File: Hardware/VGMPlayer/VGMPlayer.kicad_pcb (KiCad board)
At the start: 2 copper layers, 94.5 x 103.1 mm, 141 parts, among them J1 Barrel_Jack_Switch, J2 Conn_01x20_Male, J3 Conn_01x20_Male, J4 Conn_01x20_Male, J5 Conn_01x20_Male, U1 STC8951, U10 LTC6903, U11 HC-06, U2 7805-VGM, U3 LM386, U4 LM386, U5 OLED_128_64_I2C, U6 AUDIOJACK-VGM, U7 YM2612, U8 SN76489, U9 LTC6903, Y1 11.0592MHz

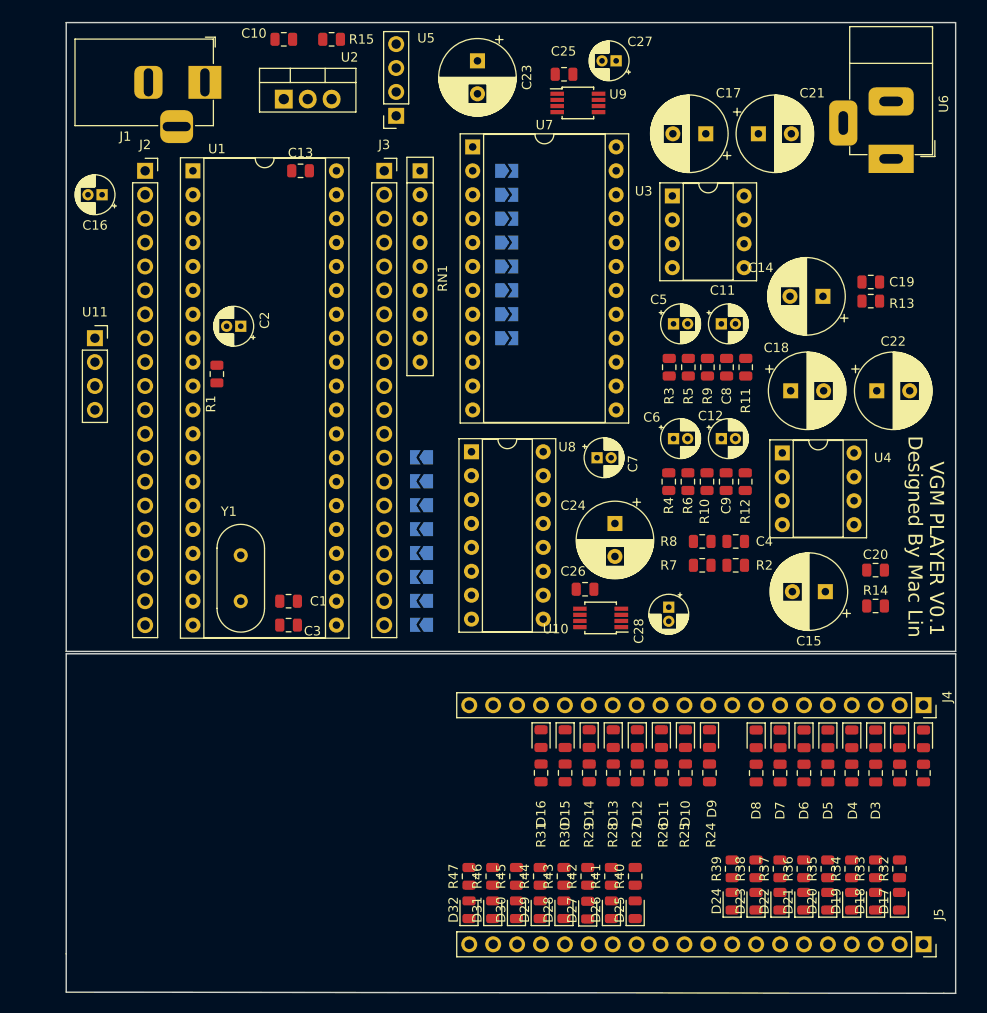
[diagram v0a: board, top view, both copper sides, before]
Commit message: 1
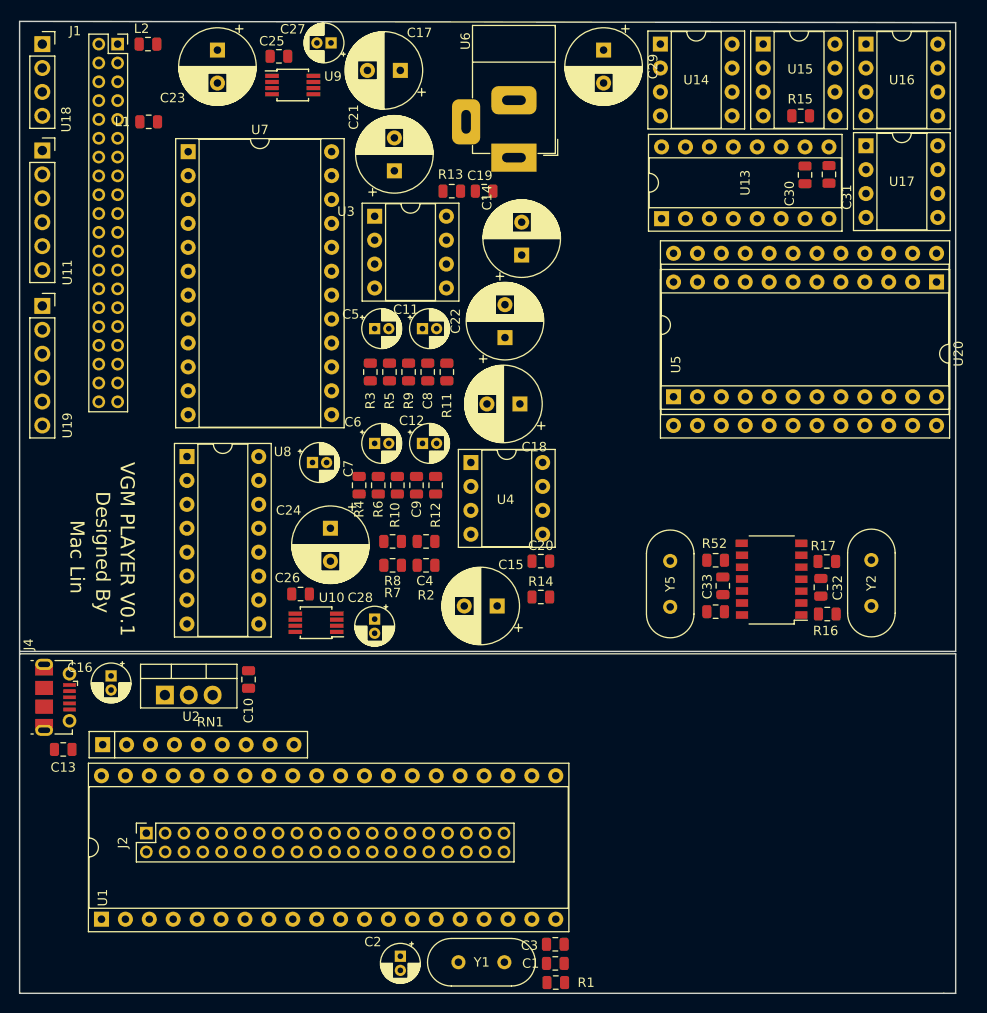
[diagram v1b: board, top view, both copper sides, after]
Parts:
- removed D1, D10, D11, D12, D13, D14, D15, D16, D17, D18, D19, D2, D20, D21, D22, D23, D24, D25, D26, D27, D28, D29, D3, D30, D31, D32, D4, D5, D6, D7, D8, D9: LED, LED_SMD:LED_0805_2012Metric
- removed J3, J5: Conn_01x20_Male, Connector_PinSocket_2.54mm:PinSocket_1x20_P2.54mm_Vertical
- removed JP1, JP10, JP11, JP12, JP13, JP14, JP15, JP16, JP2, JP3, JP4, JP5, JP6, JP7, JP8, JP9: Jumper_NC_Small, Jumper:SolderJumper-2_P1.3mm_Open_TrianglePad1.0x1.5mm
- removed R18, R19, R20, R21, R22, R23, R24, R25, R26, R27, R28, R29, R30, R31, R32, R33, R34, R35, R36, R37, R38, R39, R40, R41, R42, R43, R44, R45, R46, R47: 1k, Resistor_SMD:R_0805_2012Metric
- added C29: 10uF, Capacitor_THT:CP_Radial_D8.0mm_P3.50mm, F.Cu at (109.9, 63.4)
- added C30: 1.5nF, Capacitor_SMD:C_0805_2012Metric, F.Cu at (131.3, 76.6)
- added C31: 1.5nF, Capacitor_SMD:C_0805_2012Metric, F.Cu at (133.9, 76.6)
- added C32: 33pF, Capacitor_SMD:C_0805_2012Metric, F.Cu at (133.0, 120.4)
- added C33: 33pF, Capacitor_SMD:C_0805_2012Metric, F.Cu at (122.6, 120.3)
- added L1: L, Inductor_SMD:L_0805_2012Metric, F.Cu at (61.6, 71.0)
- added L2: L, Inductor_SMD:L_0805_2012Metric, F.Cu at (61.5, 62.7)
- added R51: 1k, Resistor_SMD:R_0805_2012Metric, F.Cu at (121.8, 123.0)
- added R52: 1k, Resistor_SMD:R_0805_2012Metric, F.Cu at (121.8, 117.6)
- added U12: 74HC04, VGM:SOP-14_4.4x8.3mm_P1.27mm, F.Cu at (127.8, 118.9)
- added U13: YM3012, Package_DIP:DIP-16_W7.62mm_Socket, F.Cu at (116.1, 81.3)
- added U14: LM386, Package_DIP:DIP-8_W7.62mm_Socket, F.Cu at (116.0, 62.7)
- added U15: LM386, Package_DIP:DIP-8_W7.62mm_Socket, F.Cu at (126.9, 62.7)
- added U16: LM386, Package_DIP:DIP-8_W7.62mm_Socket, F.Cu at (137.8, 62.7)
- added U17: LM386, Package_DIP:DIP-8_W7.62mm_Socket, F.Cu at (137.8, 73.5)
- added U18: OLED_128_64_I2C, Connector_PinSocket_2.54mm:PinSocket_1x04_P2.54mm_Vertical, F.Cu at (50.3, 62.7)
- added U19: ESP8266Module, Connector_PinSocket_2.54mm:PinSocket_1x06_P2.54mm_Vertical, F.Cu at (50.3, 90.6)
- added U20: YM2612, Package_DIP:DIP-24_W15.24mm_Socket, F.Cu at (145.3, 88.0)
- added Y2: 3.768Mhz, Crystal:Crystal_HC49-4H_Vertical, F.Cu at (138.4, 122.4)
- added Y5: 7.67Mhz, Crystal:Crystal_HC49-4H_Vertical, F.Cu at (117.0, 122.5)
- J1: value Barrel_Jack_Switch -> Conn_02x20_Odd_Even; footprint Connector_BarrelJack:BarrelJack_Horizontal -> Connector_PinSocket_2.00mm:PinSocket_2x20_P2.00mm_Vertical
- J2: value Conn_01x20_Male -> Conn_02x20_Odd_Even; footprint Connector_PinSocket_2.54mm:PinSocket_1x20_P2.54mm_Vertical -> Connector_PinSocket_2.00mm:PinSocket_2x20_P2.00mm_Vertical
- J4: value Conn_01x20_Male -> USB_B_Micro; footprint Connector_PinSocket_2.54mm:PinSocket_1x20_P2.54mm_Vertical -> Connector_USB:USB_Micro-B_Molex-105017-0001
- R15: value 0 -> 270
- U11: footprint Connector_PinSocket_2.54mm:PinSocket_1x04_P2.54mm_Vertical -> Connector_PinSocket_2.54mm:PinSocket_1x06_P2.54mm_Vertical
- U5: value OLED_128_64_I2C -> YM2151; footprint Connector_PinSocket_2.54mm:PinSocket_1x04_P2.54mm_Vertical -> Package_DIP:DIP-24_W15.24mm_Socket
- moved J4 92.2 mm to (51.7, 132.1)
- moved U1 80.1 mm to (56.6, 155.7), turned to 90 degrees
- moved R1 74.0 mm to (104.8, 162.4), turned to 0 degrees
- moved J2 70.4 mm to (61.3, 146.6), turned to 90 degrees
- moved RN1 69.7 mm to (56.7, 137.2), turned to 0 degrees
- moved C2 69.0 mm to (88.3, 159.6), turned to 270 degrees
- moved C10 68.1 mm to (72.2, 130.2), turned to 270 degrees
- moved C13 66.4 mm to (52.5, 137.7), turned to 180 degrees
- moved U2 64.6 mm to (63.3, 131.9)
- moved C16 51.1 mm to (57.6, 129.9), turned to 270 degrees
- moved R15 50.5 mm to (130.9, 70.4), turned to 180 degrees
- moved Y1 49.0 mm to (94.5, 160.3), turned to 0 degrees
- moved C1 47.8 mm to (104.8, 160.4)
- moved R13 46.0 mm to (93.8, 78.4), turned to 180 degrees
- moved C3 44.2 mm to (104.8, 158.4)
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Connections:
- net Net-(U10-Pad6) renamed SN_CLK
- net Net-(U7-Pad24) renamed YM_CLK
- C1 pad 1: GND -> GND_8051
- C1 pad 2: XTAL2 -> Net-(C1-Pad2)
- C10 pad 1: GND -> GND_8051
- C10 pad 2: +5V -> +5V_8051
- C13 pad 1: VCC -> +5V_8051
- C13 pad 2: GND -> GND_8051
- C14 pad 1: VCC -> +5V
- C14 pad 2: GND -> GNDA
- C15 pad 1: VCC -> +5V
- C15 pad 2: GND -> GNDA
- C16 pad 1: VCC -> Net-(C16-Pad1)
- C16 pad 2: GND -> GND_8051
- C17 pad 2: GND -> GNDA
- C18 pad 2: GND -> GNDA
- C2 pad 1: VCC -> +5V_8051
- C2 pad 2: RST -> Net-(C2-Pad2)
- C23 pad 1: VCC -> VDD
- C24 pad 1: VCC -> VDD
- C25 pad 2: VCC -> VDD
- C26 pad 2: VCC -> VDD
- C27 pad 1: VCC -> VDD
- C28 pad 1: VCC -> VDD
- C3 pad 1: GND -> GND_8051
- C3 pad 2: XTAL1 -> Net-(C3-Pad2)
- C4 pad 2: GND -> GNDA
- J1 pad 1: +5V -> Net-(J1-Pad1)
- J1 pad 2: GND -> +5V
- J1 pad 3: Net-(J1-Pad3) -> D0
- J2 pad 1: YM_D0 -> +3V3_8051
- J2 pad 10: RXD -> P0.1
- J2 pad 11: TXD -> P1.3
- J2 pad 12: YM_CS -> P2.7
- J2 pad 13: YM_WR -> P1.4
- J2 pad 14: YM_RD -> GND_8051
- J2 pad 15: YM_A0 -> P1.5
- J2 pad 16: YM_A1 -> P2.6
- J2 pad 17: YM_IC -> +3V3_8051
- J2 pad 18: XTAL2 -> P2.5
- J2 pad 19: XTAL1 -> P1.6
- J2 pad 2: YM_D1 -> +5V_8051
- J2 pad 20: GND -> GND_8051
- J2 pad 3: YM_D2 -> P1.0
- J2 pad 4: YM_D3 -> +5V_8051
- J2 pad 5: YM_D4 -> P1.1
- J2 pad 6: YM_D5 -> GND_8051
- J2 pad 7: YM_D6 -> P1.2
- J2 pad 8: YM_D7 -> P0.0
- J2 pad 9: RST -> GND_8051
- J4 pad 1: Net-(D1-Pad1) -> Net-(C16-Pad1)
- J4 pad 5: Net-(D5-Pad1) -> GND_8051
- J4 pad 6: Net-(D6-Pad1) -> GND_8051
- R1 pad 1: RST -> Net-(C2-Pad2)
- R1 pad 2: GND -> GND_8051
- R13 pad 2: GND -> GNDA
- R14 pad 2: GND -> GNDA
- R15 pad 1: VCC -> Net-(R15-Pad1)
- R15 pad 2: +5V -> Net-(R15-Pad2)
- R16 pad 2: Net-(J5-Pad1) -> Net-(R16-Pad2)
- R17 pad 2: Net-(J5-Pad1) -> Net-(C32-Pad1)
- R2 pad 1: GND -> GNDA
- R3 pad 1: GND -> GNDA
- R4 pad 1: GND -> GNDA
- RN1 pad 1: VCC -> +5V_8051
- RN1 pad 2: I2C_SCK -> P0.0
- RN1 pad 3: I2C_SDA -> P0.1
- RN1 pad 4: SN_WR -> P0.2
- U1 pad 1: YM_D0 -> P1.0
- U1 pad 10: RXD -> P3.0
- U1 pad 11: TXD -> P3.1
- U1 pad 12: YM_CS -> P3.2
- U1 pad 13: YM_WR -> P3.3
- U1 pad 14: YM_RD -> P3.4
- U1 pad 15: YM_A0 -> P3.5
- U1 pad 16: YM_A1 -> P3.6
- U1 pad 17: YM_IC -> P3.7
- U1 pad 18: XTAL2 -> Net-(C1-Pad2)
- U1 pad 19: XTAL1 -> Net-(C3-Pad2)
- U1 pad 2: YM_D1 -> P1.1
- U1 pad 20: GND -> GND_8051
- U1 pad 29: PSEN -> Net-(U1-Pad29)
- U1 pad 3: YM_D2 -> P1.2
- U1 pad 30: ALE -> Net-(U1-Pad30)
- U1 pad 31: VCC -> +5V_8051
- U1 pad 37: SN_WR -> P0.2
- U1 pad 38: I2C_SDA -> P0.1
- U1 pad 39: I2C_SCK -> P0.0
- U1 pad 4: YM_D3 -> P1.3
- U1 pad 40: VCC -> +5V_8051
- U1 pad 5: YM_D4 -> P1.4
- U1 pad 6: YM_D5 -> P1.5
- U1 pad 7: YM_D6 -> P1.6
- U1 pad 8: YM_D7 -> P1.7
- U1 pad 9: RST -> Net-(C2-Pad2)
- U10 pad 2: IIC_SDA -> I2C_SDA
- U10 pad 3: IIC_SCK -> I2C_SCK
- U10 pad 7: VCC -> VDD
- U10 pad 8: VCC -> VDD
- U11 pad 1: VCC -> Net-(U11-Pad1)
- U11 pad 2: GND -> VDD
- U11 pad 3: RXD -> GND
- U11 pad 4: TXD -> RXD
- U2 pad 1: +5V -> +5V_8051
- U2 pad 2: GND -> GND_8051
- U2 pad 3: VCC -> Net-(C16-Pad1)
- U3 pad 2: GND -> GNDA
- U3 pad 4: GND -> GNDA
- U3 pad 6: VCC -> +5V
- U4 pad 2: GND -> GNDA
- U4 pad 4: GND -> GNDA
- U4 pad 6: VCC -> +5V
- U5 pad 1: GND -> GND_YM2151
- U5 pad 2: VCC -> YM2151_IRQ
- U5 pad 3: I2C_SCK -> YM2151_IC
- U5 pad 4: I2C_SDA -> YM2151_A0
- U6 pad 3: GND -> GNDA
- U7 pad 19: GND -> GNDA
- U7 pad 2: YM_D0 -> D0
- U7 pad 22: VCC -> +5V
- U7 pad 23: VCC -> VDD
- U7 pad 3: YM_D1 -> D1
- U7 pad 4: YM_D2 -> D2
- U7 pad 5: YM_D3 -> D3
- U7 pad 6: YM_D4 -> D4
- U7 pad 7: YM_D5 -> D5
- U7 pad 8: YM_D6 -> D6
- U7 pad 9: YM_D7 -> D7
- U8 pad 1: SN_D5 -> D5
- U8 pad 10: SN_D0 -> D0
- U8 pad 11: SN_D1 -> D1
- U8 pad 12: SN_D2 -> D2
- U8 pad 13: SN_D3 -> D3
- U8 pad 15: SN_D4 -> D4
- U8 pad 16: VCC -> VDD
- U8 pad 2: SN_D6 -> D6
- U8 pad 3: SN_D7 -> D7
- U9 pad 2: IIC_SDA -> I2C_SDA
- U9 pad 3: IIC_SCK -> I2C_SCK
- U9 pad 7: VCC -> VDD
- U9 pad 8: VCC -> VDD
- Y1 pad 1: XTAL2 -> Net-(C1-Pad2)
- Y1 pad 2: XTAL1 -> Net-(C3-Pad2)
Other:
- board size 94.5 x 103.1 mm -> 99.4 x 103.3 mm
- board text added: "Designed By"
- board text added: "Mac Lin"
- board text removed: "Designed By Mac Lin"
